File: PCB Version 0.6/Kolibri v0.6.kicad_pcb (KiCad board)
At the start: 8 copper layers, 29.4 x 29.4 mm, 201 parts, among them IC1 SX1280IMLTRT, IC5 LMR38025SDRRR, IC6 LMR38025SDRRR, J1 USB_C_Receptacle_USB2.0_16P, J3 Conn_Coaxial_Small, J5 Conn_01x08_MountingPin, J6 Conn_01x06_MountingPin, J7 Conn_01x06_MountingPin, Q1 BSS138, U1 RP2350A, U10 W25Q16JVUXIQ, U11 LPS22HB, U12 ICM-42688-P, U2 C5250982, U3 ESP32-C3, U4 TPS2116DRL, U5 AT7456E, U6 MT29F2G01ABAGDWB-IT:G, U7 TPS746-3.3DRV, U8 C3029047, Y1 Crystal_GND24, Y2 Crystal_GND24, Y4 Crystal_GND24, Y5 Crystal_GND24

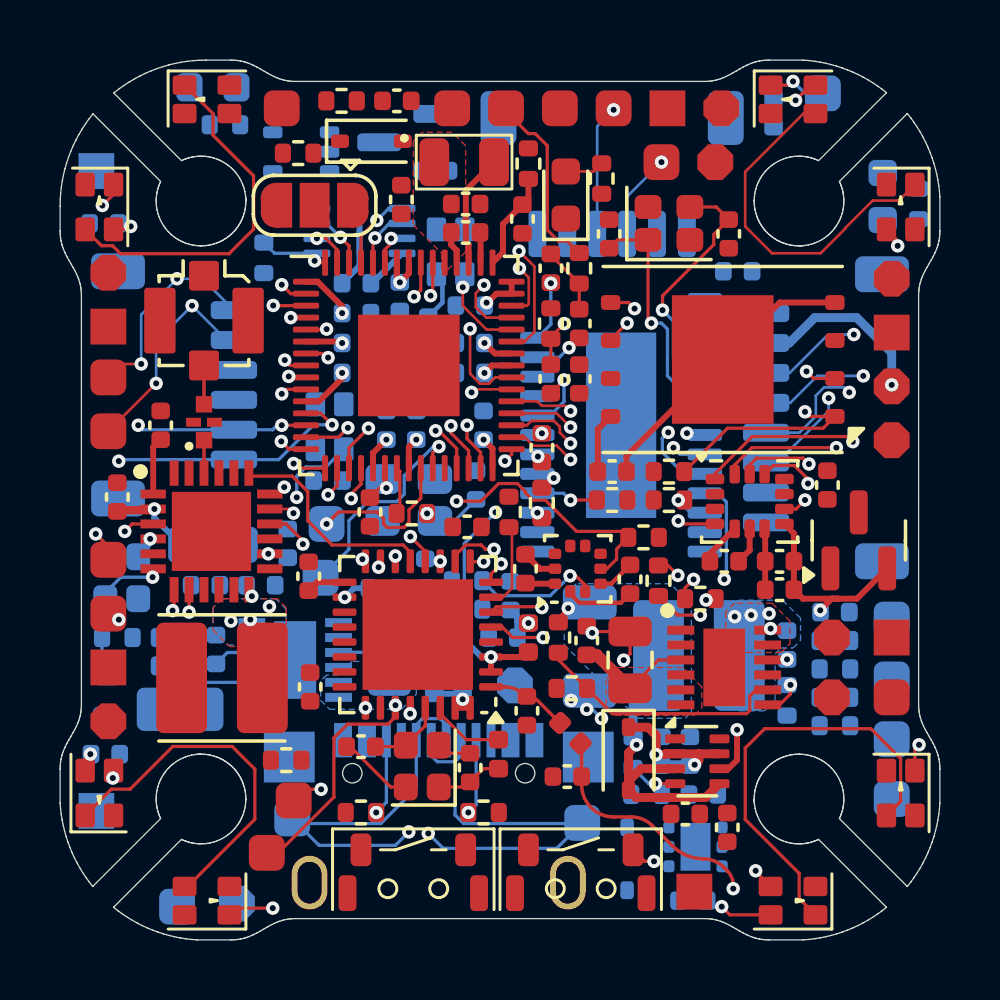
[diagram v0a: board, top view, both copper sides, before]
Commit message: wip
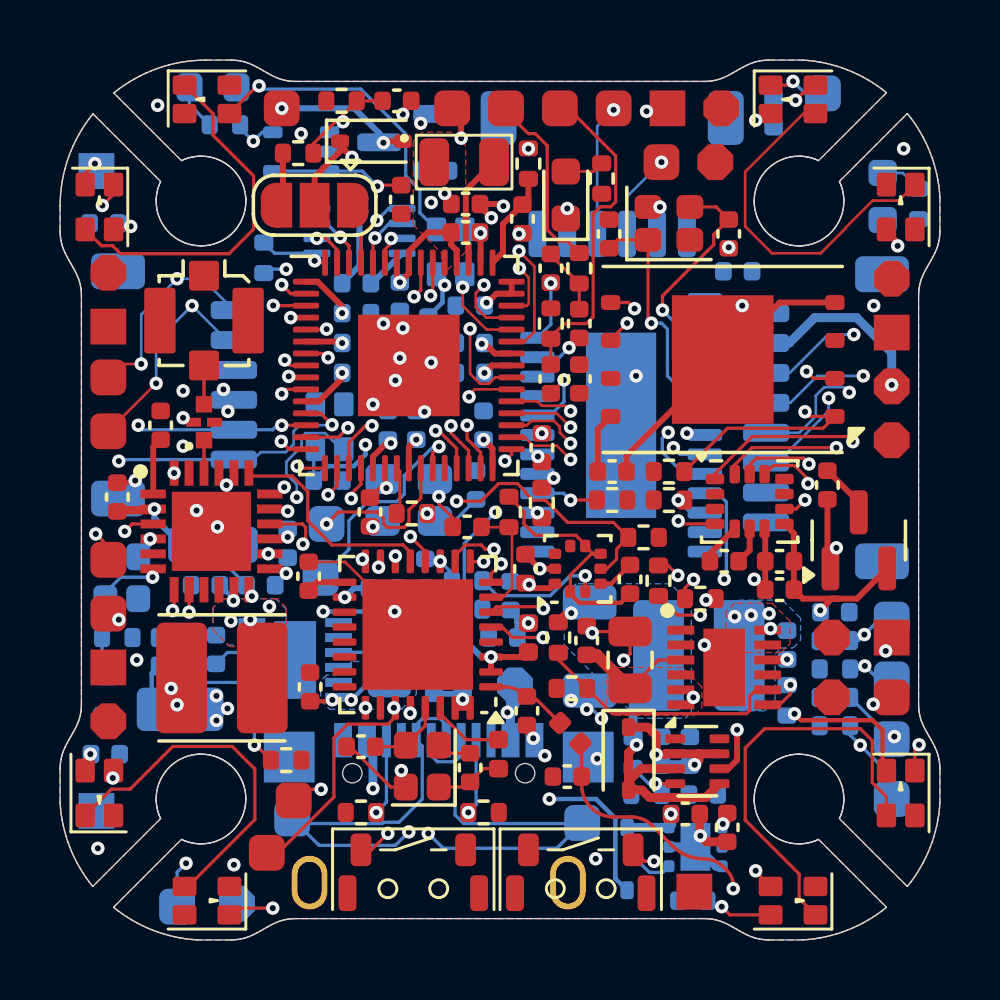
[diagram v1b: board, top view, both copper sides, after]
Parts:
- moved C69 0.05 mm to (96.3, 105.2)
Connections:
- C81 pad 2: Net-(U2-GND) -> GND
- C88 pad 2: Net-(U2-GND) -> GND
- P37 pad 1: /Connectors/PWM.1 -> /PWM.2
- P38 pad 1: /Connectors/PWM.2 -> /PWM.1
- U2 pad 1: Net-(U2-GND) -> GND
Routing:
- net +4V5: track 1.70 -> 35.7 mm, vias 0 -> 3
- net GND: track 27.1 -> 55.2 mm, vias 6 -> 63
- net Net-(R33-Pad2): track 0.00 -> 24.2 mm, vias 0 -> 2
- net /PWM.1: track 0.13 -> 20.3 mm, vias 1 -> 2
- net /U2.TX: track 5.91 -> 25.5 mm
- net /RP2350/Speaker: track 3.81 -> 23.3 mm, vias 1 -> 2
- net /U2.RX: track 3.81 -> 21.9 mm
- net /Motor.4: track 17.1 -> 33.3 mm, vias 2 -> 3
- net /Motor.3: track 18.6 -> 33.9 mm, vias 2 -> 3
- net +3V3: track 26.1 -> 39.1 mm, vias 13 -> 19
- net /ADC/VBat_ADC: track 1.92 -> 14.1 mm, vias 1 -> 2
- net /Motor.1: track 16.1 -> 28.2 mm, vias 2 -> 3
- net /Motor.2: track 17.5 -> 29.1 mm, vias 2 -> 3
- net Net-(D1-DOUT): track 0.00 -> 10.6 mm, vias 0 -> 1
- net /PWM.2: track 0.00 -> 9.75 mm, vias 1 -> 2
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- added copper zone on In2.Cu, net +1V1
- added copper zone on In3.Cu, net +3V3
- added copper zone on B.Cu, net GND
- added copper zone on F.Cu, net GND
- added copper zone on In1.Cu, net GND
- added copper zone on In2.Cu, net GND
- added copper zone on In4.Cu, net GND
- added copper zone on In5.Cu, net GND
